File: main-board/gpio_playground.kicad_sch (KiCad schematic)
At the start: 30 parts, among them SW4 SW_Push, SW6 SW_Push, SW7 SW_Push, U17 74AHC244, U18 74AHCT1G08, U19 74AHCT1G08, U20 74AHC1G04

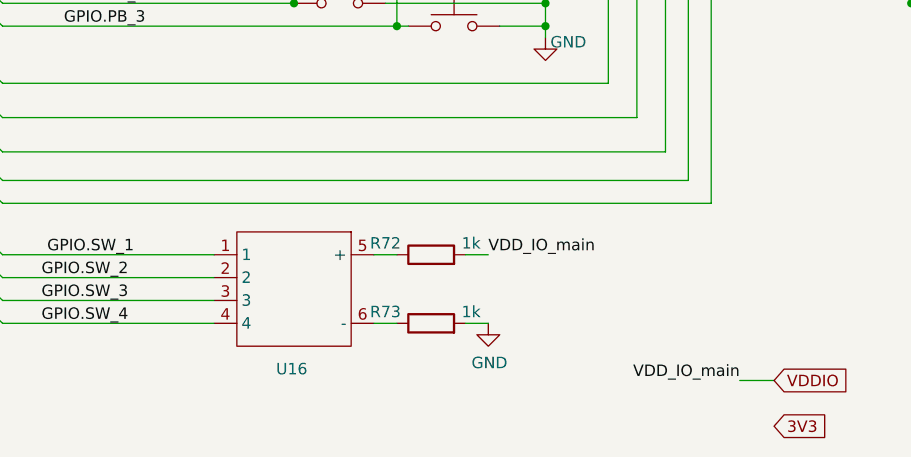
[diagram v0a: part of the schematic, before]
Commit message: pcb update
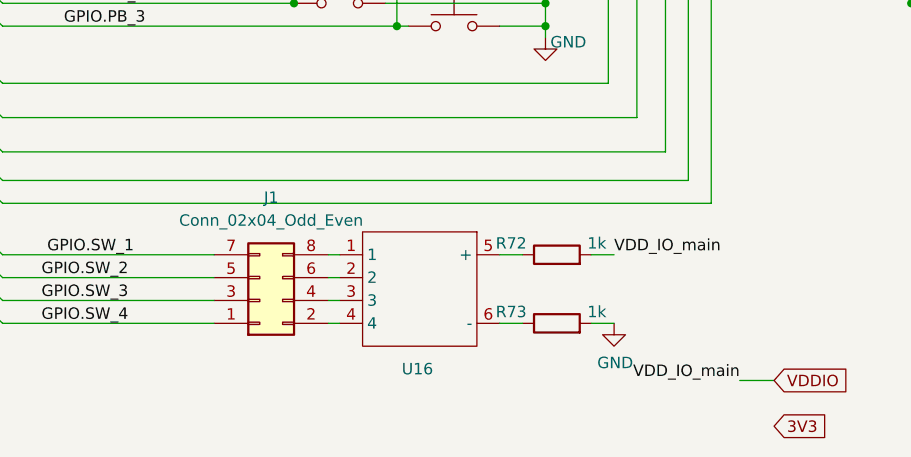
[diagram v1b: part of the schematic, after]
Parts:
- added J1: Conn_02x04_Odd_Even, Connector_PinHeader_2.54mm:PinHeader_2x04_P2.54mm_Vertical_SMD, symbol Connector_Generic:Conn_02x04_Odd_Even
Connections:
- net GPIO.SW_1: now also J1.7 (Pin_7); no longer U16.1
- net GPIO.SW_2: now also J1.5 (Pin_5); no longer U16.2
- net GPIO.SW_3: now also J1.3 (Pin_3); no longer U16.3
- net GPIO.SW_4: now also J1.1 (Pin_1); no longer U16.4
- new net: J1.2 (Pin_2), U16.4
- new net: J1.4 (Pin_4), U16.3
- new net: J1.6 (Pin_6), U16.2
- new net: J1.8 (Pin_8), U16.1
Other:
- moved on the sheet: R72, R73, U16
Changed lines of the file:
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@@
 	(wire
 		(pts
-			(xy 116.84 166.37) (xy 114.3 166.37)
+			(xy 130.81 166.37) (xy 128.27 166.37)
 		)
 		(stroke
@@
 	(wire
 		(pts
+			(xy 109.22 166.37) (xy 110.49 166.37)
+		)
+		(stroke
+			(width 0)
+			(type default)
+		)
+	)
+	(wire
+		(pts
 			(xy 213.995 113.03) (xy 210.82 113.03)
 		)
@@
 	(wire
 		(pts
-			(xy 124.46 158.75) (xy 127 158.75)
+			(xy 138.43 158.75) (xy 140.97 158.75)
 		)
 		(stroke
@@
 	(wire
 		(pts
+			(xy 109.22 163.83) (xy 110.49 163.83)
+		)
+		(stroke
+			(width 0)
+			(type default)
+		)
+	)
+	(wire
+		(pts
 			(xy 116.84 114.3) (xy 116.84 115.57)
 		)
@@
 	(wire
 		(pts
-			(xy 116.84 158.75) (xy 114.3 158.75)
+			(xy 130.81 158.75) (xy 128.27 158.75)
 		)
 		(stroke
@@
 	(wire
 		(pts
-			(xy 124.46 166.37) (xy 127 166.37)
+			(xy 138.43 166.37) (xy 140.97 166.37)
 		)
 		(stroke
@@
 	(wire
 		(pts
+			(xy 109.22 158.75) (xy 110.49 158.75)
+		)
+		(stroke
+			(width 0)
+			(type default)
+		)
+	)
+	(wire
+		(pts
 			(xy 105.41 114.3) (xy 116.84 114.3)
 		)
@@
 		)
 	)
+	(wire
+		(pts
+			(xy 109.22 161.29) (xy 110.49 161.29)
+		)
+		(stroke
+			(width 0)
+			(type default)
+		)
+	)
 	(label "GPIO.PB_1"
 		(at 88.9 128.27 180)
@@
 	)
 	(label "VDD_IO_main"
-		(at 127 158.75 0)
+		(at 140.97 158.75 0)
 		(effects
 			(font
@@
 	(symbol
 		(lib_id "Device:R")
-		(at 120.65 166.37 90)
+		(at 134.62 166.37 90)
 		(unit 1)
 		(exclude_from_sim no)
@@
 		(dnp no)
 		(property "Reference" "R73"
-			(at 115.57 165.1 90)
+			(at 129.54 165.1 90)
 			(effects
 				(font
@@
 		)
 		(property "Value" "1k"
-			(at 125.095 165.1 90)
+			(at 139.065 165.1 90)
 			(effects
 				(font
@@
 		)
 		(property "Footprint" "Resistor_SMD:R_0603_1608Metric"
-			(at 120.65 168.148 90)
+			(at 134.62 168.148 90)
 			(effects
 				(font
@@
 		)
 		(property "Datasheet" "~"
-			(at 120.65 166.37 0)
+			(at 134.62 166.37 0)
 			(effects
 				(font
@@
 		)
 		(property "Description" ""
-			(at 120.65 166.37 0)
+			(at 134.62 166.37 0)
 			(effects
 				(font
@@
 		)
 		(property "LCSC" "C21190"
-			(at 120.65 161.29 0)
+			(at 134.62 161.29 0)
 			(effects
 				(font
@@
 	)
 	(symbol
+		(lib_id "Connector_Generic:Conn_02x04_Odd_Even")
+		(at 101.6 163.83 0)
+		(mirror x)
+		(unit 1)
+		(exclude_from_sim no)
+		(in_bom yes)
+		(on_board yes)
+		(dnp no)
+		(property "Reference" "J1"
+			(at 102.87 152.4 0)
+			(effects
+				(font
+					(size 1.27 1.27)
+				)
+			)
+		)
+		(property "Value" "Conn_02x04_Odd_Even"
+			(at 102.87 154.94 0)
+			(effects
+				(font
+					(size 1.27 1.27)
+				)
+			)
+		)
+		(property "Footprint" "Connector_PinHeader_2.54mm:PinHeader_2x04_P2.54mm_Vertical_SMD"
+			(at 101.6 163.83 0)
+			(effects
+				(font
+					(size 1.27 1.27)
+				)
+				(hide yes)
+			)
+		)
+		(property "Datasheet" "~"
+			(at 101.6 163.83 0)
+			(effects
+				(font
+					(size 1.27 1.27)
+				)
+				(hide yes)
+			)
+		)
+		(property "Description" "Generic connector, double row, 02x04, odd/even pin numbering scheme (row 1 odd numbers, row 2 even numbers), script generated (kicad-library-utils/schlib/autogen/connector/)"
+			(at 101.6 163.83 0)
+			(effects
+				(font
+					(size 1.27 1.27)
+				)
+				(hide yes)
+			)
+		)
+		(pin "2"
+		)
+		(pin "7"
+		)
+		(pin "4"
+		)
+		(pin "1"
+		)
+		(pin "5"
+		)
+		(pin "3"
+		)
+		(pin "8"
+		)
+		(pin "6"
+		)
+		(instances
+			(project ""
+				(path "/6198f783-b154-4adf-87fa-b1d9cb913fe2/fd9da62b-9782-45f1-a1dc-4f8db8879f00"
+					(reference "J1")
+					(unit 1)
+				)
+			)
+		)
+	)
+	(symbol
 		(lib_id "Device:R")
 		(at 207.01 118.11 90)
@@
 	(symbol
 		(lib_id "cheeps-tb:SPDT-4bit-tri-state")
-		(at 111.76 168.91 0)
+		(at 125.73 168.91 0)
 		(mirror y)
 		(unit 1)
@@
 		(dnp no)
 		(property "Reference" "U16"
-			(at 105.156 171.45 0)
+			(at 119.126 171.45 0)
 			(effects
 				(font
@@
 		)
 		(property "Value" "~"
-			(at 105.41 154.94 0)
+			(at 119.38 154.94 0)
 			(effects
 				(font
@@
 		)
 		(property "Footprint" "heep_footprints:BIWIN_DTS04GE_SMD"
-			(at 111.76 168.91 0)
+			(at 125.73 168.91 0)
 			(effects
 				(font
@@
 		)
 		(property "Datasheet" "https://www.lcsc.com/datasheet/C3294670.pdf"
-			(at 111.76 168.91 0)
+			(at 125.73 168.91 0)
 			(effects
 				(font
@@
 		)
 		(property "Description" ""
-			(at 111.76 168.91 0)
+			(at 125.73 168.91 0)
 			(effects
 				(font
@@
 	(symbol
 		(lib_id "power:GND")
-		(at 127 166.37 0)
+		(at 140.97 166.37 0)
 		(unit 1)
 		(exclude_from_sim no)
@@
 		(dnp no)
 		(property "Reference" "#PWR11"
-			(at 127 172.72 0)
+			(at 140.97 172.72 0)
 			(effects
 				(font
@@
 		)
 		(property "Value" "GND"
-			(at 127.127 170.7642 0)
+			(at 141.097 170.7642 0)
 			(effects
 				(font
@@
 		)
 		(property "Footprint" ""
-			(at 127 166.37 0)
+			(at 140.97 166.37 0)
 			(effects
 				(font
@@
 		)
 		(property "Datasheet" ""
-			(at 127 166.37 0)
+			(at 140.97 166.37 0)
 			(effects
 				(font
@@
 		)
 		(property "Description" "Power symbol creates a global label with name \"GND\" , ground"
-			(at 127 166.37 0)
+			(at 140.97 166.37 0)
 			(effects
 				(font
@@
 	(symbol
 		(lib_id "Device:R")
-		(at 120.65 158.75 90)
+		(at 134.62 158.75 90)
 		(unit 1)
 		(exclude_from_sim no)
@@
 		(dnp no)
 		(property "Reference" "R72"
-			(at 115.57 157.48 90)
+			(at 129.54 157.48 90)
 			(effects
 				(font
@@
 		)
 		(property "Value" "1k"
-			(at 125.095 157.48 90)
+			(at 139.065 157.48 90)
 			(effects
 				(font
@@
 		)
 		(property "Footprint" "Resistor_SMD:R_0603_1608Metric"
-			(at 120.65 160.528 90)
+			(at 134.62 160.528 90)
 			(effects
 				(font
@@
 		)
 		(property "Datasheet" "~"
-			(at 120.65 158.75 0)
+			(at 134.62 158.75 0)
 			(effects
 				(font
@@
 		)
 		(property "Description" ""
-			(at 120.65 158.75 0)
+			(at 134.62 158.75 0)
 			(effects
 				(font
@@
 		)
 		(property "LCSC" "C21190"
-			(at 120.65 153.67 0)
+			(at 134.62 153.67 0)
 			(effects
 				(font
